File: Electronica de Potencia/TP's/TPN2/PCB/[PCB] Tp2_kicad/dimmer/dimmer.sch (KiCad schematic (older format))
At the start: 17 parts, among them J1 Conn_01x02, J2 Conn_01x02, Q1 2N2646, Q2 TIC106

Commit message: Modularizo el proyecto para que sea portable para cualquiera, completo 3d's, me falta conseguir la Res de 5W para ver si corresponde el fp
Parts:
- added G1: LOGO, lib_fp:logo_utn_fsilk_small, symbol logo:LOGO
- added RV1, RV2: R_POT_TRIM, lib_fp:Potentiometer_Bourns_3266Y_Vertical, symbol dimmer_sch:Device_R_POT_TRIM
- C1: footprint Capacitor_THT:C_Rect_L13.5mm_W5.0mm_P10.00mm_FKS3_FKP3_MKS4 -> lib_fp:C_Rect_L13.5mm_W5.0mm_P10.00mm_FKS3_FKP3_MKS4; symbol Device:C -> dimmer_sch:Device_C
- D1: footprint Diode_THT:D_DO-41_SOD81_P10.16mm_Horizontal -> lib_fp:D_DO-41_SOD81_P10.16mm_Horizontal; symbol Diode:1N4007 -> dimmer_sch:Diode_1N4007
- D2, D3, D4, D5: footprint Diode_THT:D_DO-41_SOD81_P10.16mm_Horizontal -> lib_fp:D_DO-41_SOD81_P10.16mm_Horizontal; symbol Diode:1N4007 -> dimmer_sch:1N4007
- DZ1: footprint Diode_THT:D_DO-41_SOD81_P10.16mm_Horizontal -> lib_fp:D_DO-41_SOD81_P10.16mm_Horizontal; symbol Diode:1N47xxA -> dimmer_sch:1N47xxA
- F1: footprint Fuse_Holders_and_Fuses:Fuseholder5x20_horiz_SemiClosed_Casing10x25mm -> lib_fp:Fuseholder5x20_horiz_SemiClosed_Casing10x25mm; symbol Device:Fuse -> dimmer_sch:Device_Fuse
- J1, J2: footprint TerminalBlock:TerminalBlock_bornier-2_P5.08mm -> lib_fp:TerminalBlock_bornier-2_P5.08mm; symbol Connector_Generic:Conn_01x02 -> dimmer_sch:Connector_Generic_Conn_01x02
- Q1: footprint Package_TO_SOT_THT:TO-18-3 -> lib_fp:TO-18-3; symbol Transistor_BJT:2N2646 -> dimmer_sch:Transistor_BJT_2N2646
- Q2: footprint Package_TO_SOT_THT:TO-220-3_Vertical -> lib_fp:TO-220-3_Vertical; symbol Triac_Thyristor:TIC106 -> dimmer_sch:Triac_Thyristor_TIC106
- R1: footprint Resistor_THT:R_Axial_Shunt_L22.2mm_W8.0mm_PS14.30mm_P25.40mm -> lib_fp:R_Axial_Shunt_L22.2mm_W8.0mm_PS14.30mm_P25.40mm; symbol Device:R -> dimmer_sch:Device_R_US
- R2: footprint Potentiometer_THT:Potentiometer_Alps_RK163_Single_Horizontal -> lib_fp:Potentiometer_Alps_RK163_Single_Horizontal; symbol Device:R_POT -> dimmer_sch:Device_R_POT
- R3, R4, R5: footprint Resistor_THT:R_Axial_DIN0207_L6.3mm_D2.5mm_P10.16mm_Horizontal -> lib_fp:R_Axial_DIN0207_L6.3mm_D2.5mm_P10.16mm_Horizontal; symbol Device:R_US -> dimmer_sch:Device_R_US
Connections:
- net labels added: power_GND
- net labels removed: GND

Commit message: Arreglo footprint de UJT
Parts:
- removed Q1: 2N2646, lib_fp:TO-18-3, symbol dimmer_sch:Transistor_BJT_2N2646
- added Q1: 2N2647, lib_fp:TO-18-3, symbol dimmer_sch:2N2647
- G1: symbol logo:LOGO -> dimmer-rescue:LOGO-logo
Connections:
- net at D3.1 (K), D4.1 (K), R1.1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: now also Q2.2 (A)
- net at C1.1, D5.1 (K), R5.2: now also Q1.1 (E)
- net at R3.2: now also Q1.3 (B2)
- net at Q2.3 (G), R4.1: now also Q1.2 (B1)
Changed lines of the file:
@@
 Connection ~ 6350 4550
-$Comp
-L dimmer_sch:Transistor_BJT_2N2646 Q1
-U 1 1 5CB53134
-P 7600 4000
-F 0 "Q1" H 7790 4046 50  0000 L CNN
-F 1 "2N2646" H 7790 3955 50  0000 L CNN
-F 2 "lib_fp:TO-18-3" H 7800 3925 50  0001 L CIN
-F 3 "http://www.bucek.name/pdf/2n2646,2647.pdf" H 7600 4000 50  0001 L CNN
-	1    7600 4000
-	1    0    0    -1
-$EndComp
 $Comp
 L dimmer_sch:Device_R_US R3
@@
 Wire Wire Line
 	7150 4550 8350 4550
-Wire Wire Line
-	8350 3000 8350 4050
 $Comp
 L dimmer_sch:Connector_Generic_Conn_01x02 J2
@@
 $EndComp
 $Comp
-L logo:LOGO G1
+L dimmer-rescue:LOGO-logo G1
 U 1 1 5CB4E2BD
 P 3500 4800
@@
 	1    0    0    -1
 $EndComp
+Wire Wire Line
+	8350 4000 8350 3000
+$Comp
+L dimmer_sch:2N2647 Q1
+U 1 1 5CB52F99
+P 7600 4000
+F 0 "Q1" H 7790 4046 50  0000 L CNN
+F 1 "2N2647" H 7790 3955 50  0000 L CNN
+F 2 "lib_fp:TO-18-3" H 7800 3925 50  0001 L CIN
+F 3 "" H 7600 4000 50  0001 L CNN
+	1    7600 4000
+	1    0    0    -1
+$EndComp

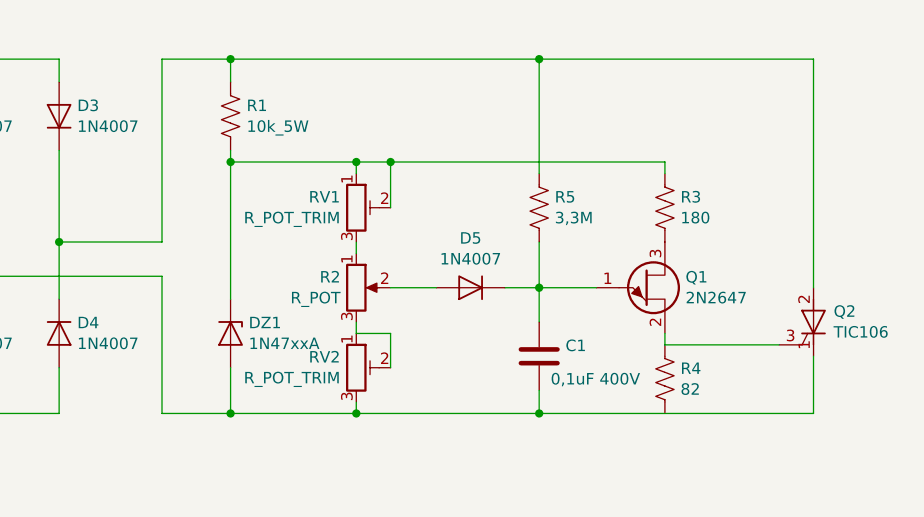
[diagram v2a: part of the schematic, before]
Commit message: Arreglando a little bit
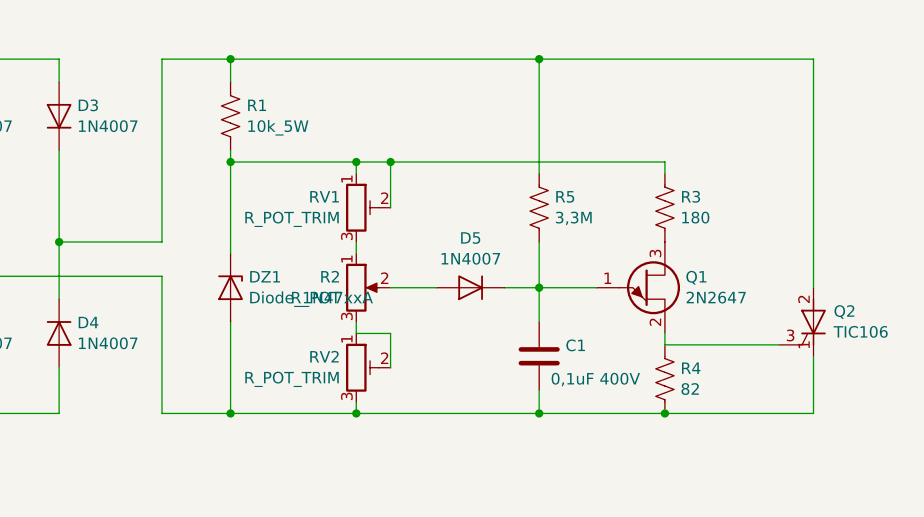
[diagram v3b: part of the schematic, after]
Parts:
- removed DZ1: 1N47xxA, lib_fp:D_DO-41_SOD81_P10.16mm_Horizontal, symbol dimmer_sch:1N47xxA
- added DZ1: Diode_1N47xxA, lib_fp:D_DO-41_SOD81_P10.16mm_Horizontal, symbol dimmer_sch:Diode_1N47xxA
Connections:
- net at C1.2, D1.2 (A), D2.2 (A)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: now also R4.2, DZ1.2 (A)
- net at R1.2, R3.1, RV1.1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: now also DZ1.1 (K)
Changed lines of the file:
@@
 Wire Wire Line
 	5800 3100 5800 3000
-$Comp
-L dimmer_sch:1N47xxA DZ1
-U 1 1 5CB48759
-P 5800 4200
-F 0 "DZ1" V 5754 4279 50  0000 L CNN
-F 1 "1N47xxA" V 5845 4279 50  0000 L CNN
-F 2 "lib_fp:D_DO-41_SOD81_P10.16mm_Horizontal" H 5800 4025 50  0001 C CNN
-F 3 "https://www.vishay.com/docs/85816/1n4728a.pdf" H 5800 4200 50  0001 C CNN
-	1    5800 4200
-	0    1    1    0
-$EndComp
-Wire Wire Line
-	5800 4050 5800 3450
-Wire Wire Line
-	5800 4550 5500 4550
 Wire Wire Line
 	5500 4550 5500 3950
 Wire Wire Line
 	5500 3950 4500 3950
-Wire Wire Line
-	5800 4350 5800 4550
 Connection ~ 4500 3950
 Wire Wire Line
@@
 Wire Wire Line
 	6350 3450 5800 3450
-Connection ~ 5800 3450
 Wire Wire Line
 	5800 3450 5800 3400
@@
 	-1   0    0    1
 $EndComp
-Wire Wire Line
-	6350 4550 5800 4550
-Connection ~ 5800 4550
 $Comp
 L dimmer_sch:Device_R_US R5
@@
 $EndComp
 Wire Wire Line
-	7150 4550 8350 4550
+	7150 4550 7700 4550
 $Comp
 L dimmer_sch:Connector_Generic_Conn_01x02 J2
@@
 	1    0    0    -1
 $EndComp
+Wire Wire Line
+	5500 4550 5800 4550
+$Comp
+L dimmer_sch:Diode_1N47xxA DZ1
+U 1 1 5CB5BBFF
+P 5800 4000
+F 0 "DZ1" V 5754 4079 50  0000 L CNN
+F 1 "Diode_1N47xxA" V 5845 4079 50  0000 L CNN
+F 2 "lib_fp:D_DO-41_SOD81_P10.16mm_Horizontal" H 5800 3825 50  0001 C CNN
+F 3 "" H 5800 4000 50  0001 C CNN
+	1    5800 4000
+	0    1    1    0
+$EndComp
+Wire Wire Line
+	5800 3850 5800 3450
+Connection ~ 5800 3450
+Wire Wire Line
+	5800 4150 5800 4550
+Connection ~ 5800 4550
+Wire Wire Line
+	5800 4550 6350 4550
+Connection ~ 7700 4550
+Wire Wire Line
+	7700 4550 8350 4550
 $EndSCHEMATC
